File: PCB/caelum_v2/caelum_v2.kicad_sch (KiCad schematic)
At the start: 29 parts, among them J1 Conn_01x06_Pin, J10 Conn_01x04_Pin, J3 Pulse1, J4 Batt, J6 Pulse2, J7 Conn_01x04_Pin, J8 DS18B20, Q1 FS8205A-FC, U1 DW01A, U2 MCP1700T-3302E, U3 ESP32-H2-SUPERMINI

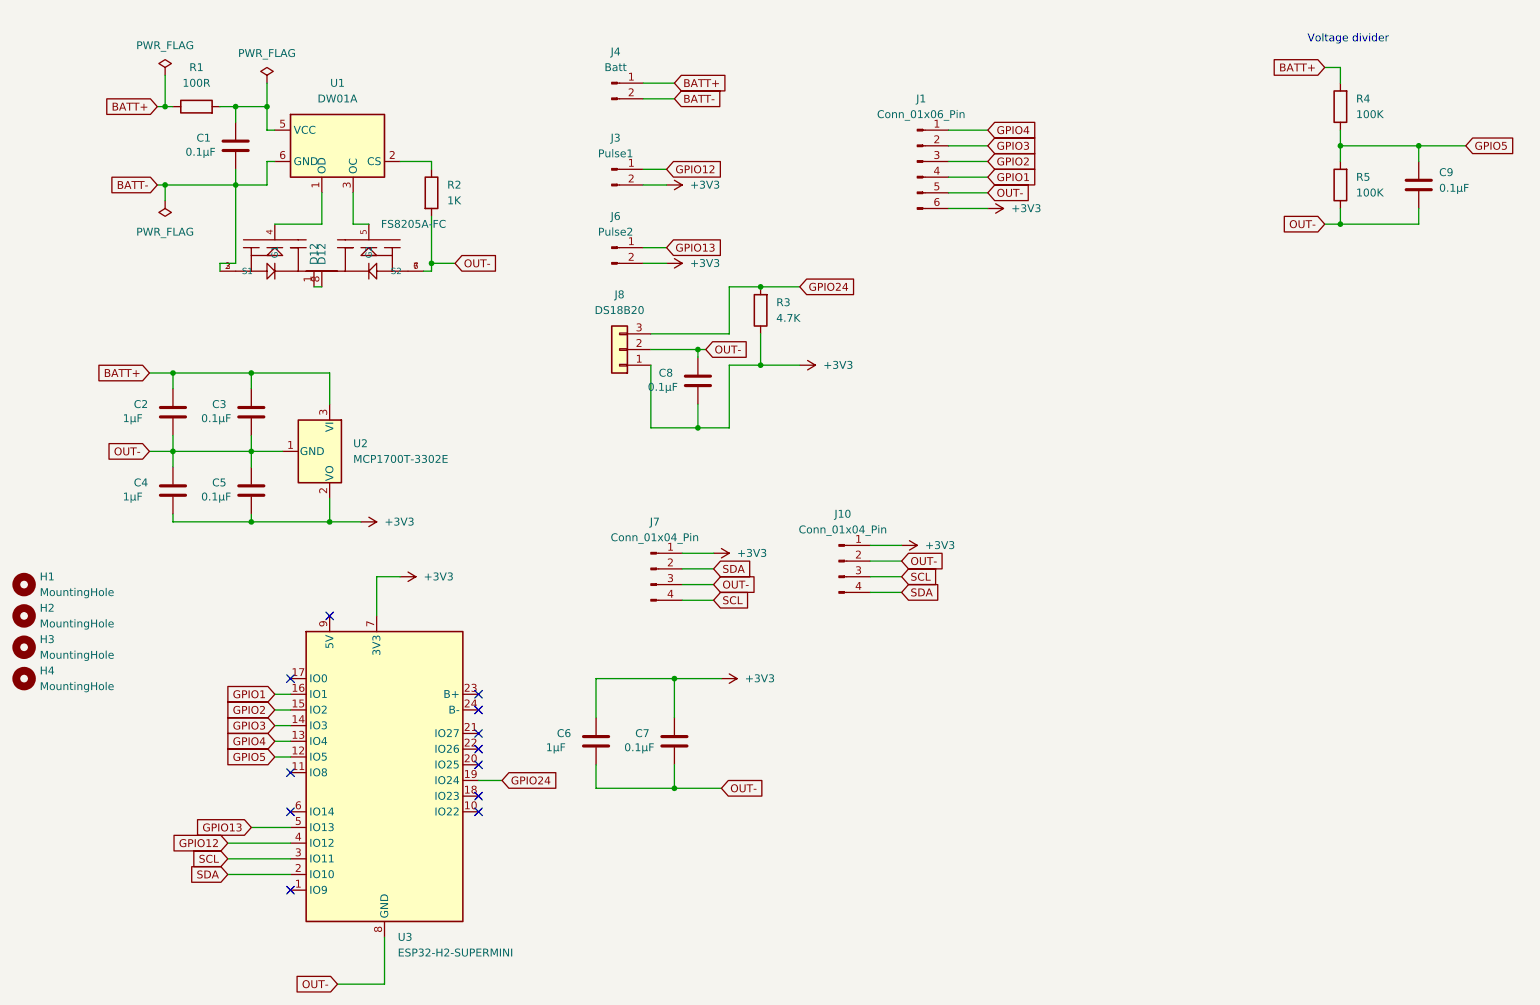
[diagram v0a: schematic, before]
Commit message: Add PCB v2
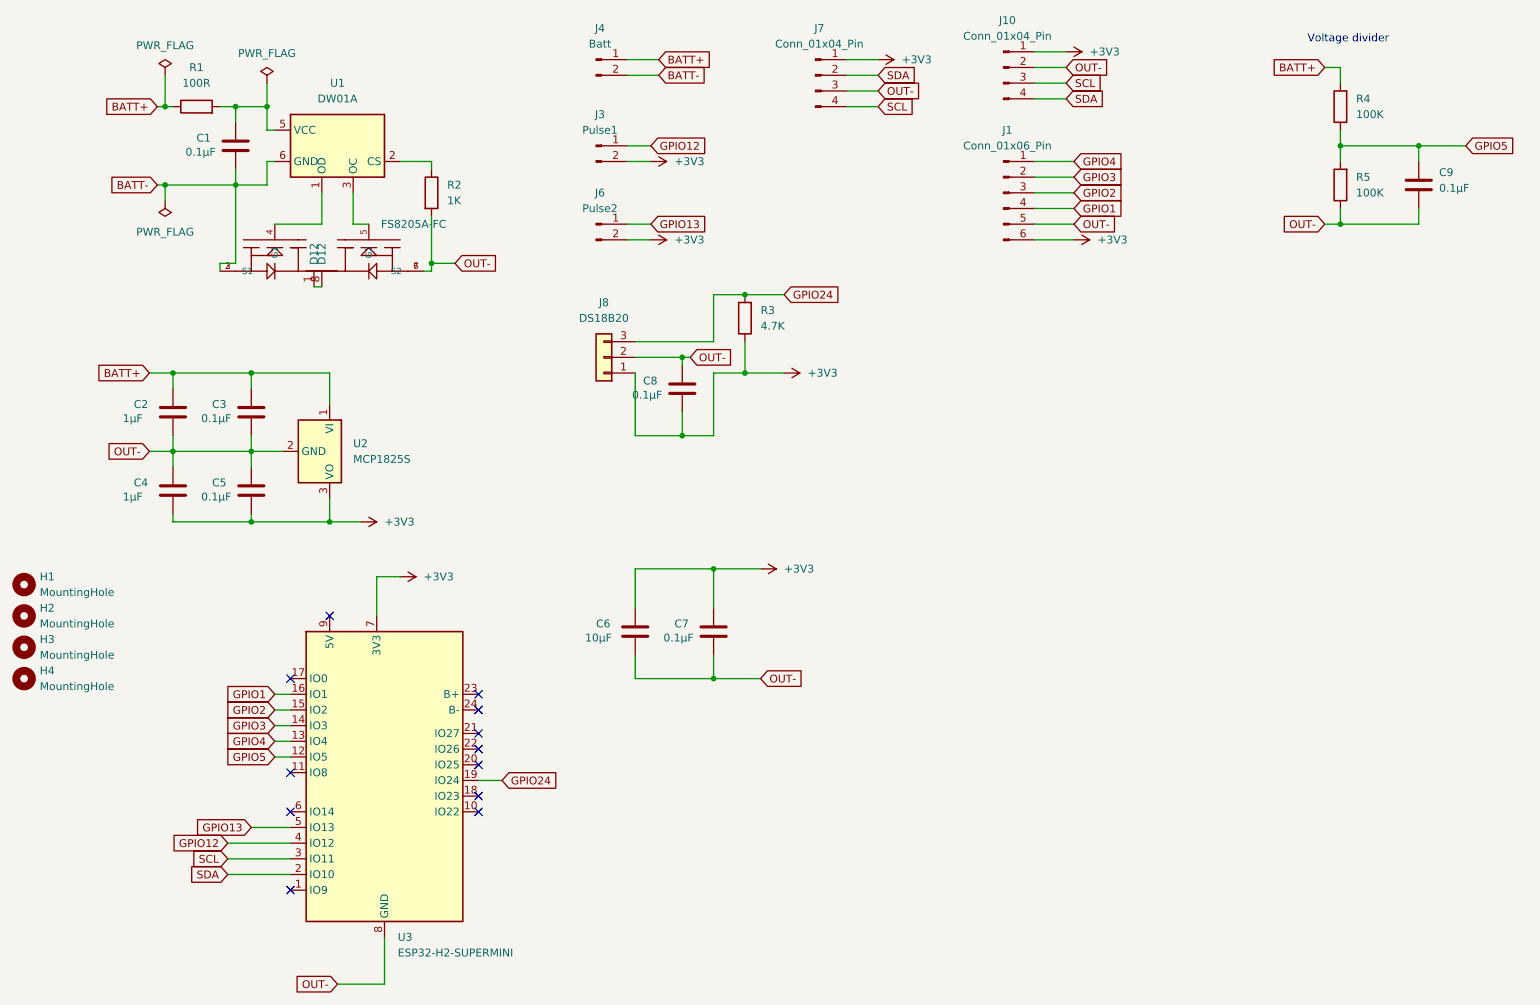
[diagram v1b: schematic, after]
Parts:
- removed U2: MCP1700T-3302E, Package_TO_SOT_SMD:SOT-23, symbol Regulator_Linear:MCP1700x-330xxTT
- added U2: MCP1825S, Package_TO_SOT_SMD:SOT-223-3_TabPin2, symbol Regulator_Linear:MCP1825S
- C6: value 1µF -> 10µF
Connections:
- net +3V3: now also U2.3 (VO)
- net BATT+: now also U2.1 (VI)
- net OUT-: now also U2.2 (GND)
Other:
- moved on the sheet: C6, C7, C8, J1, J10, J3, J4, J6, J7, J8, R3
